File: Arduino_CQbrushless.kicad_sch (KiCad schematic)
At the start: 3 parts, among them J1 Nucleo_F302R8, J2 AE-LLCNV8-DIP20

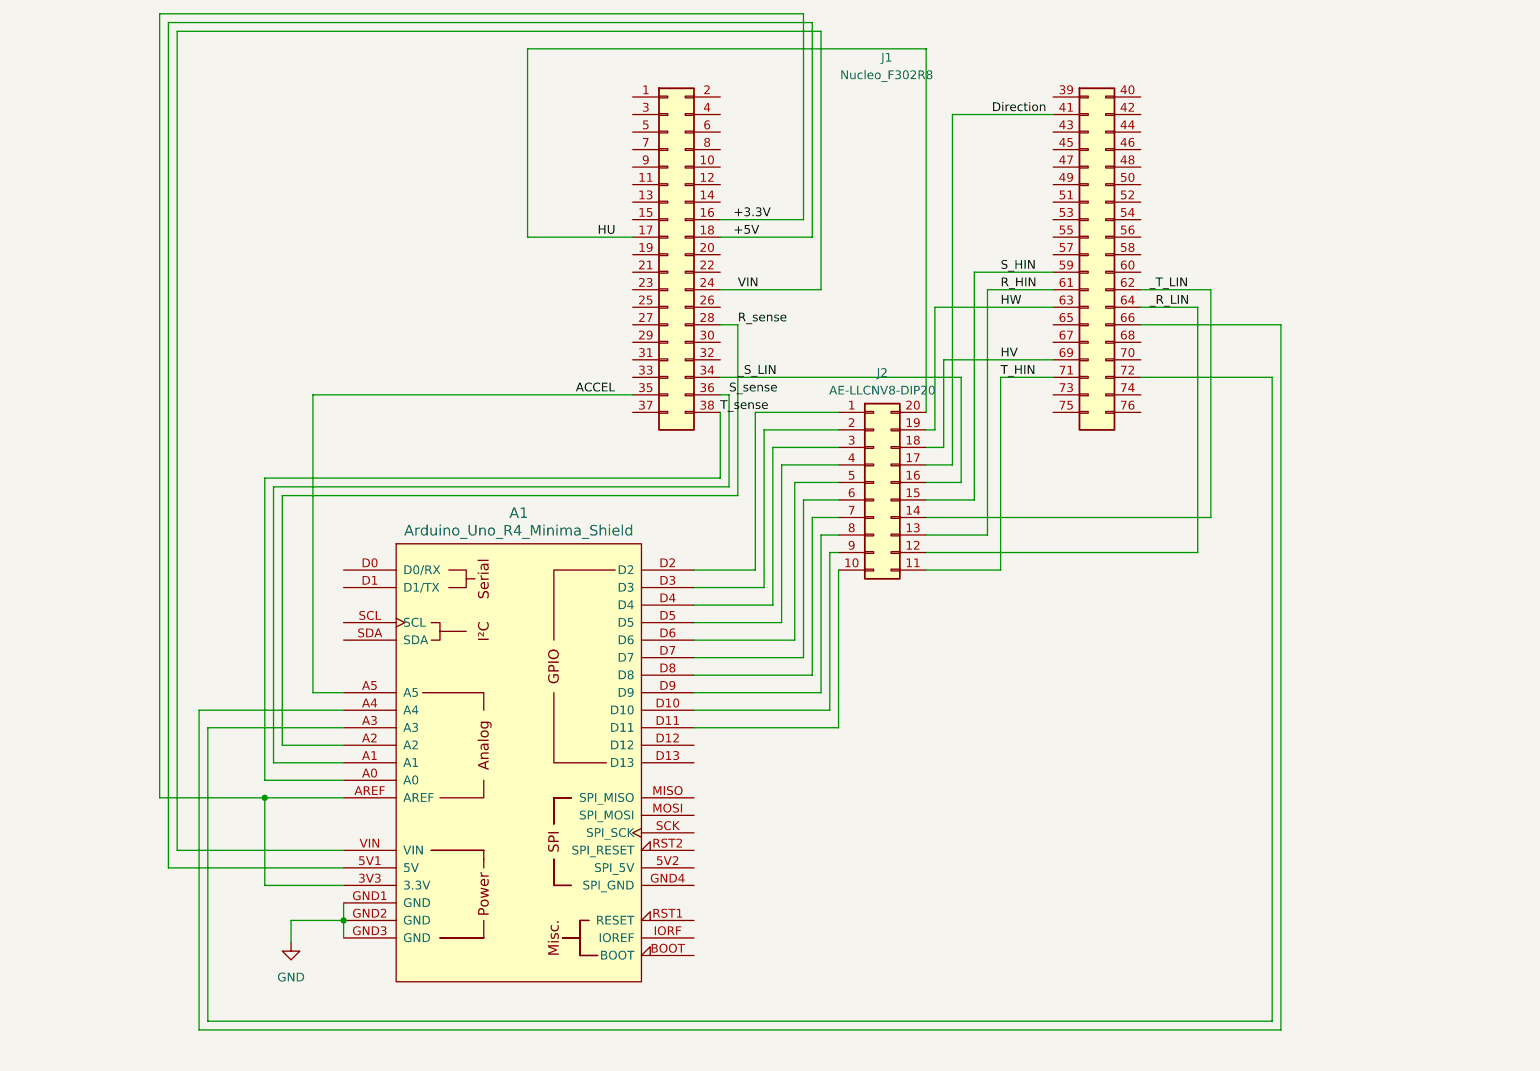
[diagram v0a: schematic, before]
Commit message: 1228
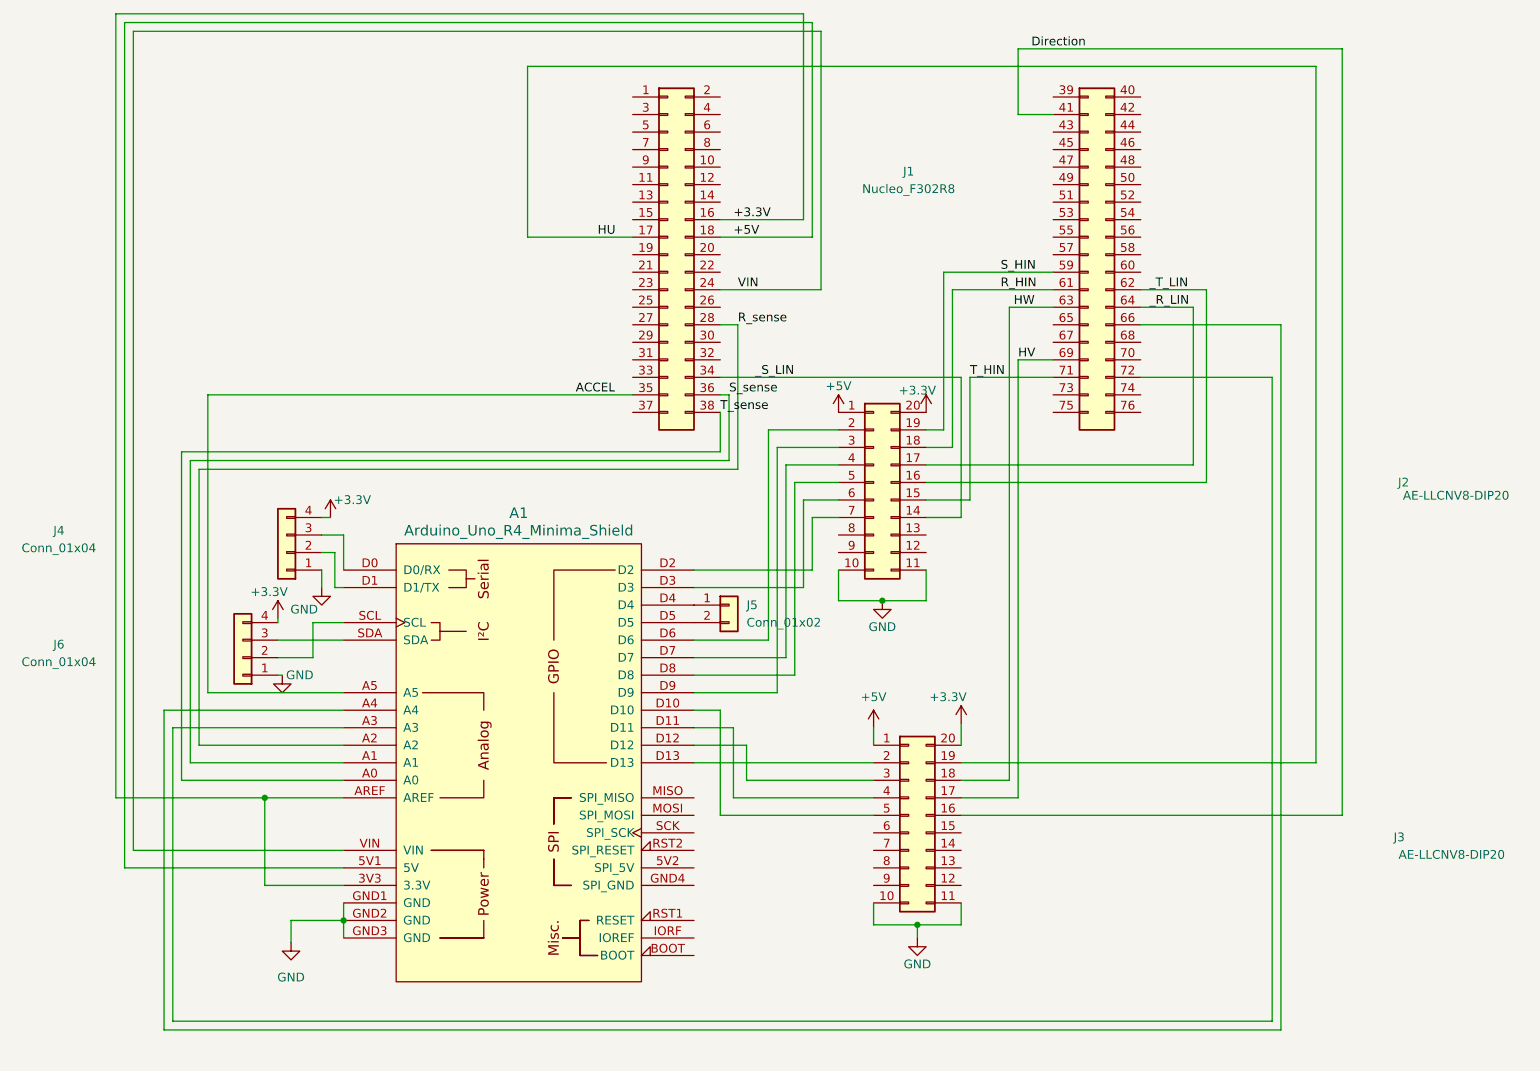
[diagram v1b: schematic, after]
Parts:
- added J3: AE-LLCNV8-DIP20, Library:AE-LLCNV8-DIP, symbol New_Library:AE-LLCNV8-DIP20
- added J4, J6: Conn_01x04, Connector_PinHeader_2.54mm:PinHeader_1x04_P2.54mm_Vertical, symbol Connector_Generic:Conn_01x04
- added J5: Conn_01x02, Connector_PinHeader_2.54mm:PinHeader_1x02_P2.54mm_Vertical, symbol Connector_Generic:Conn_01x02
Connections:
- net +3.3V: now also J2.20 (VB), J3.20 (VB), J4.4 (Pin_4), J6.4 (Pin_4)
- net +5V: now also J2.1 (VA), J3.1 (VA)
- net Direction: now also J3.16 (B3); no longer J2.17 (B2)
- net GND: now also J2.10 (GND), J2.11 (OE), J3.10 (GND), J3.11 (OE), J4.1 (Pin_1), J6.1 (Pin_1)
- net HU: now also J3.19 (B0); no longer J2.20 (VB)
- net HV: now also J3.17 (B2); no longer J2.18 (B1)
- net HW: now also J3.18 (B1); no longer J2.19 (B0)
- net R_HIN: now also J2.18 (B1); no longer J2.13 (B6)
- net R_sense: no longer J1.34 (Pin_34), J2.16 (B3)
- net S_HIN: now also J2.19 (B0); no longer J2.15 (B4)
- net T_HIN: now also J2.15 (B4); no longer J2.11 (OE)
- net _R_LIN: now also J2.17 (B2); no longer J2.12 (B7)
- net _T_LIN: now also J2.16 (B3); no longer J2.14 (B5)
- net at A1.D0 (D0/RX): now also J4.3 (Pin_3)
- net at A1.D1 (D1/TX): now also J4.2 (Pin_2)
- net at A1.D10: now also J3.5 (A3); no longer J2.9 (A7)
- net at A1.D11: now also J3.4 (A2); no longer J2.10 (GND)
- net at A1.D12: now also J3.3 (A1)
- net at A1.D13: now also J3.2 (A0)
- net at A1.D2: now also J2.7 (A5); no longer J2.1 (VA)
- net at A1.D3: now also J2.6 (A4); no longer J2.2 (A0)
- net at A1.D4: now also J5.1 (Pin_1); no longer J2.3 (A1)
- net at A1.D5: now also J5.2 (Pin_2); no longer J2.4 (A2)
- net at A1.D6: now also J2.2 (A0); no longer J2.5 (A3)
- net at A1.D7: now also J2.4 (A2); no longer J2.6 (A4)
- net at A1.D8: now also J2.5 (A3); no longer J2.7 (A5)
- net at A1.D9: now also J2.3 (A1); no longer J2.8 (A6)
- net at A1.SCL: now also J6.2 (Pin_2)
- net at A1.SDA: now also J6.3 (Pin_3)
- new net _S_LIN: J1.34 (Pin_34), J2.14 (B5)

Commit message: 0108
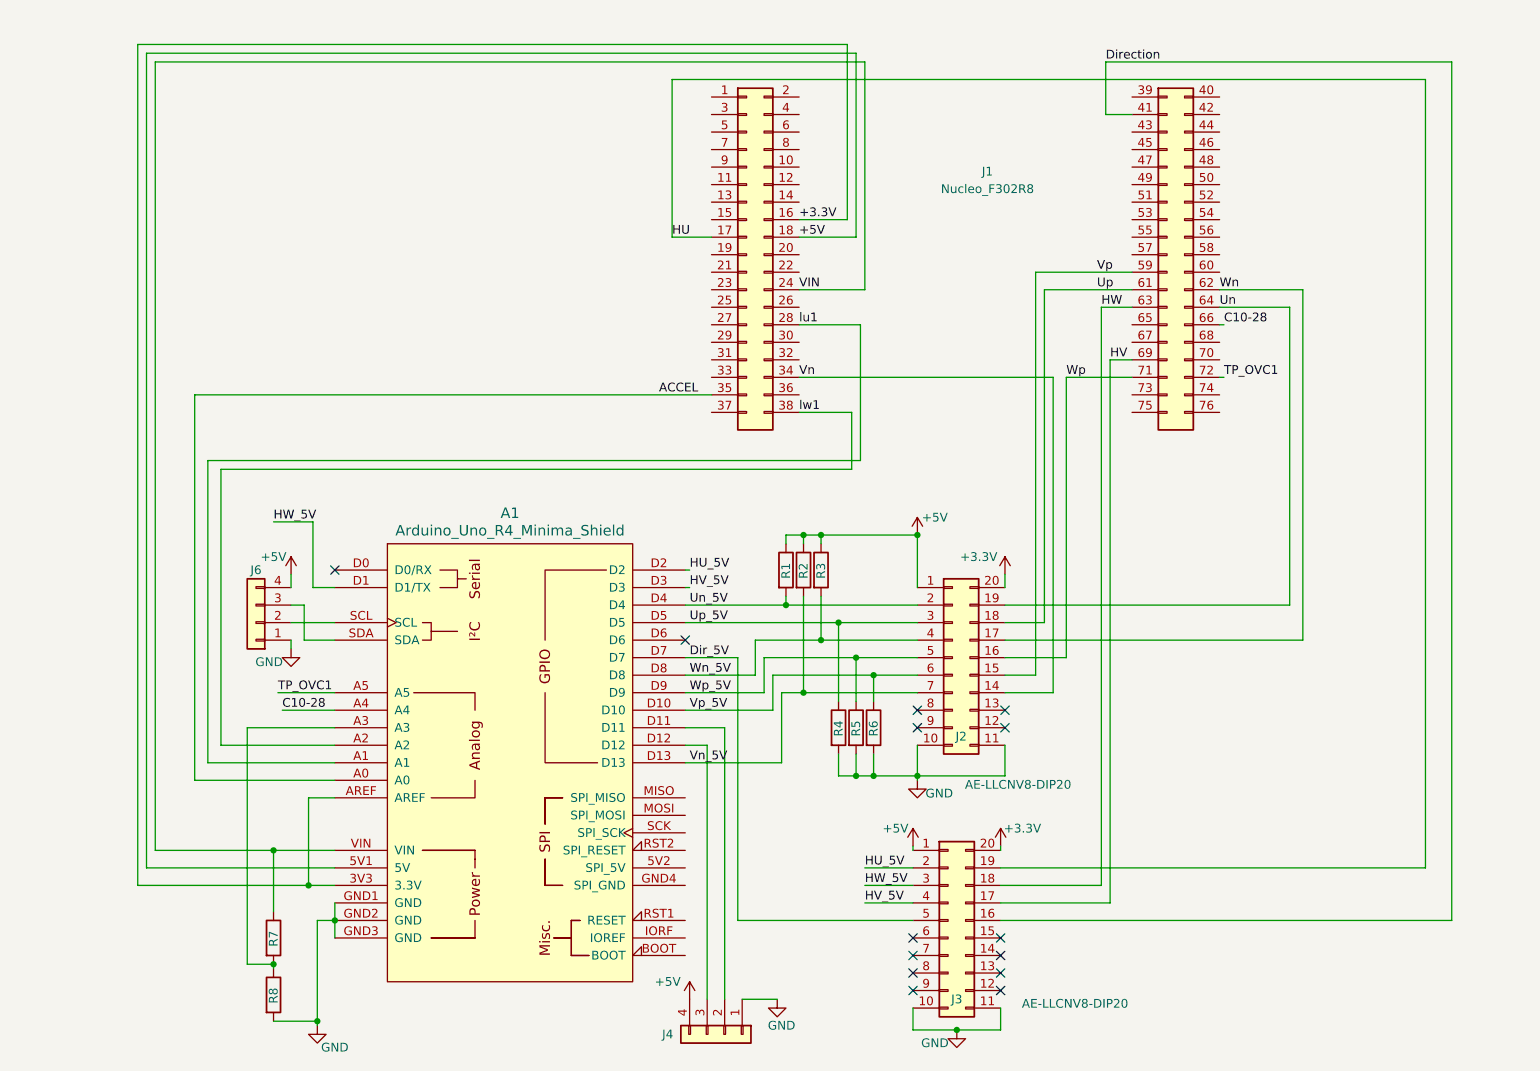
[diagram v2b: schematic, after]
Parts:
- removed J5: Conn_01x02, Connector_PinHeader_2.54mm:PinHeader_1x02_P2.54mm_Vertical, symbol Connector_Generic:Conn_01x02
- added R1, R2, R3, R4, R5, R6, R8: R, symbol Device:R
- added R7: R, Resistor_THT:R_Axial_DIN0309_L9.0mm_D3.2mm_P12.70mm_Horizontal, symbol Device:R
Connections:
- net +3.3V: no longer J4.4 (Pin_4), J6.4 (Pin_4)
- net +5V: now also J4.4 (Pin_4), J6.4 (Pin_4), R1.1, R2.1, R3.1
- net ACCEL: now also A1.A0; no longer A1.A5
- net GND: now also R4.2, R5.2, R6.2, R8.2
- net VIN: now also R7.1
- net at A1.A3: now also R7.2, R8.1; no longer J1.72
- net C10-28: now reaches A1.A4, J1.66
- net at A1.D0 (D0/RX): no longer J4.3 (Pin_3)
- net at J4.2 (Pin_2): now also A1.D11; no longer A1.D1 (D1/TX)
- net Dir_5V: now reaches J3.5 (A3)
- net Dir_5V: now also A1.D7; no longer A1.D10
- net HV_5V: now reaches J3.4 (A2)
- net HV_5V: now also A1.D3; no longer A1.D11
- net at A1.D12: now also J4.3 (Pin_3); no longer J3.3 (A1)
- net HU_5V: now reaches J3.2 (A0)
- net HU_5V: now also A1.D2; no longer A1.D13
- net Vn_5V: now reaches J2.7 (A5)
- net Vn_5V: now also A1.D13, R2.2; no longer A1.D2
- net Vp_5V: now reaches J2.6 (A4)
- net Vp_5V: now also A1.D10, R6.1; no longer A1.D3
- net Un_5V: now reaches A1.D4
- net Un_5V: now also J2.2 (A0), R1.2
- net Up_5V: now reaches A1.D5
- net Up_5V: now also J2.3 (A1), R4.1
- net at A1.D6: no longer J2.2 (A0)
- net Wn_5V: now reaches J2.4 (A2)
- net Wn_5V: now also A1.D8, R3.2; no longer A1.D7
- net Wp_5V: now reaches J2.5 (A3)
- net Wp_5V: now also A1.D9, R5.1; no longer A1.D8
- net R_HIN renamed Up
- net R_sense renamed lu1
- net lu1: now also A1.A1; no longer A1.A2
- net S_HIN renamed Un
- net Un: now also J1.64; no longer J1.59
- net S_sense: no longer names the net of J1.36 (Pin_36)
- net S_sense: no longer A1.A1
- net T_HIN renamed Vp
- net Vp: now also J1.59; no longer J1.71
- net T_sense renamed lw1
- net lw1: now also A1.A2; no longer A1.A0
- net _R_LIN renamed Wn
- net Wn: now also J1.62; no longer J1.64
- net _S_LIN renamed Vn
- net _T_LIN renamed Wp
- net Wp: now also J1.71; no longer J1.62
- new net HW_5V: A1.D1 (D1/TX), J3.3 (A1)
- new net TP_OVC1: A1.A5, J1.72
- no-connect marks 0 -> 14
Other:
- moved on the sheet: A1, J1, J2, J3, J6
